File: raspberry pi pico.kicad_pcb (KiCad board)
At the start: 2 copper layers, 51.5 x 20.6 mm, 2 parts, among them J1 USB_OTG, U1 RP2350A

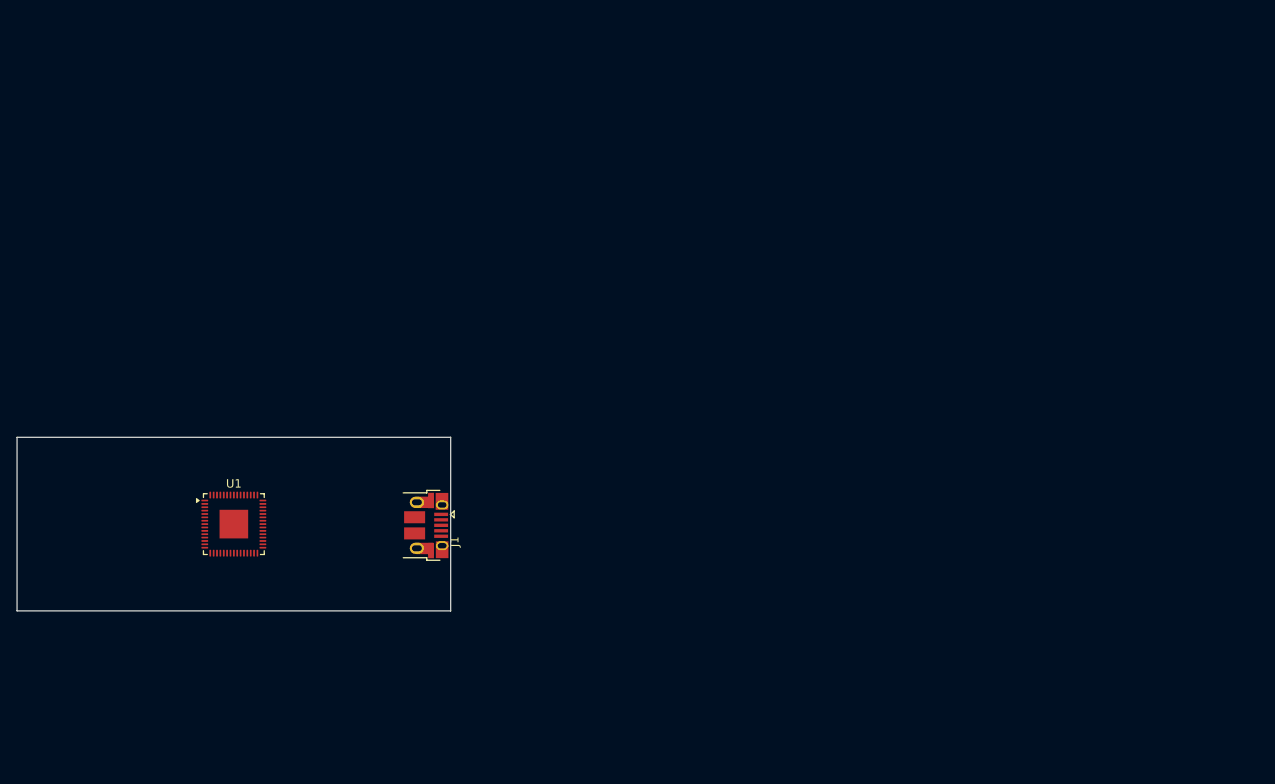
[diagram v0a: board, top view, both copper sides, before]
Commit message: Add files via upload
these files present my progress comparing to the 1st upload
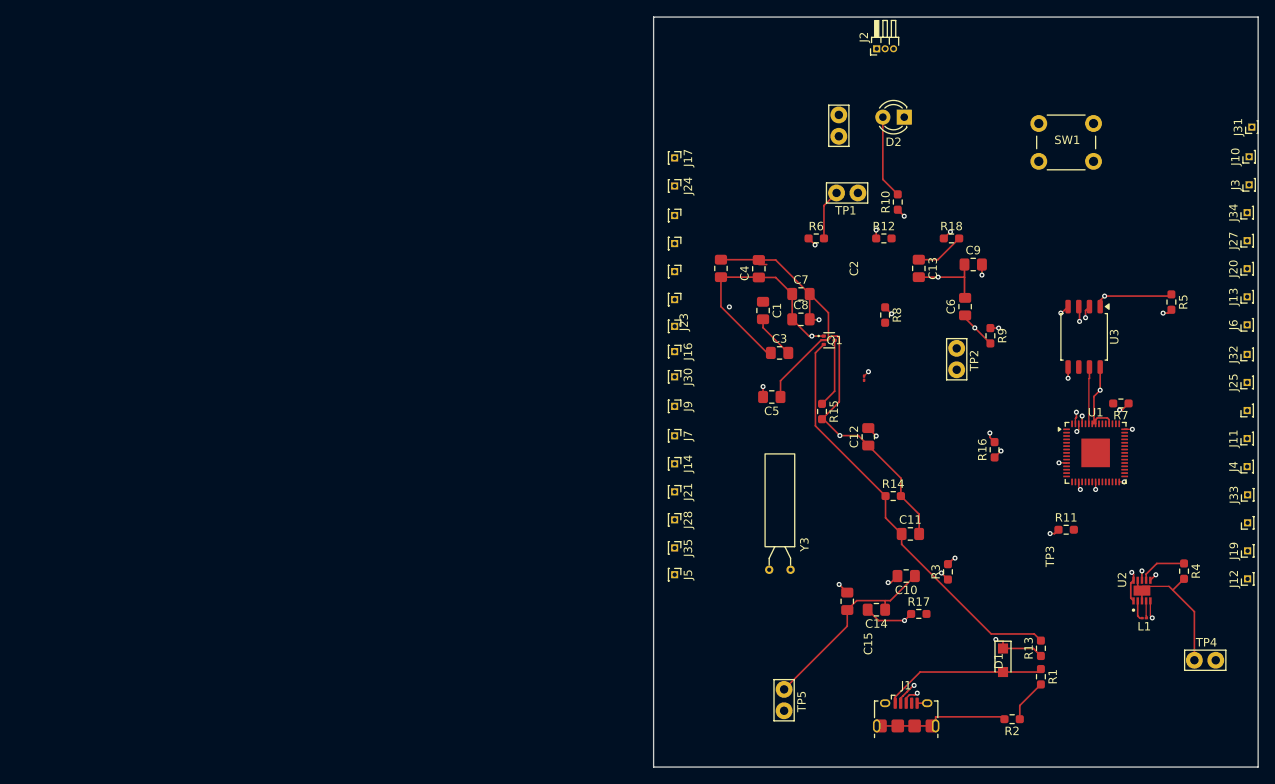
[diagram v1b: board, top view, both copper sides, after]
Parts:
- added C1: 47u, Capacitor_SMD:C_0805_2012Metric_Pad1.18x1.45mm_HandSolder, F.Cu at (213.0, 73.0)
- added C10: 4u7, Capacitor_SMD:C_0805_2012Metric_Pad1.18x1.45mm_HandSolder, F.Cu at (230.0, 104.5)
- added C11: 1n, Capacitor_SMD:C_0805_2012Metric_Pad1.18x1.45mm_HandSolder, F.Cu at (230.5, 99.5)
- added C12: 4u7, Capacitor_SMD:C_0805_2012Metric_Pad1.18x1.45mm_HandSolder, F.Cu at (225.5, 88.0)
- added C13: 4u7, Capacitor_SMD:C_0805_2012Metric_Pad1.18x1.45mm_HandSolder, F.Cu at (231.5, 68.0)
- added C14: 15p, Capacitor_SMD:C_0805_2012Metric_Pad1.18x1.45mm_HandSolder, F.Cu at (226.5, 108.5)
- added C15: 15p, Capacitor_SMD:C_0805_2012Metric_Pad1.18x1.45mm_HandSolder, F.Cu at (223.0, 107.5)
- added C2: C, Capacitor_SMD:C_0805_2012Metric_Pad1.18x1.45mm_HandSolder, F.Cu at (208.0, 68.0)
- added C3: 47uF, Capacitor_SMD:C_0805_2012Metric_Pad1.18x1.45mm_HandSolder, F.Cu at (215.0, 78.0)
- added C4: 100nF, Capacitor_SMD:C_0805_2012Metric_Pad1.18x1.45mm_HandSolder, F.Cu at (212.5, 68.0)
- added C5: 47u, Capacitor_SMD:C_0805_2012Metric_Pad1.18x1.45mm_HandSolder, F.Cu at (214.0, 83.2)
- added C6: 47u, Capacitor_SMD:C_0805_2012Metric_Pad1.18x1.45mm_HandSolder, F.Cu at (237.0, 72.5)
- added C7: 47u, Capacitor_SMD:C_0805_2012Metric_Pad1.18x1.45mm_HandSolder, F.Cu at (217.5, 71.0)
- added C8: 100nF, Capacitor_SMD:C_0805_2012Metric_Pad1.18x1.45mm_HandSolder, F.Cu at (217.5, 74.0)
- added C9: 4u7, Capacitor_SMD:C_0805_2012Metric_Pad1.18x1.45mm_HandSolder, F.Cu at (238.0, 67.5)
- added D1: PMEG6010ELR, Diode_SMD:Nexperia_CFP3_SOD-123W, F.Cu at (241.5, 114.5)
- added D2: LED, LED_THT:LED_D3.0mm, F.Cu at (229.8, 50.0)
- added J10: Conn_01x01_Pin, Connector_PinHeader_1.00mm:PinHeader_1x01_P1.00mm_Vertical, F.Cu at (270.7, 54.7)
- added J11: Conn_01x01_Pin, Connector_PinHeader_1.00mm:PinHeader_1x01_P1.00mm_Vertical, F.Cu at (270.5, 88.2)
- added J12: Conn_01x01_Pin, Connector_PinHeader_1.00mm:PinHeader_1x01_P1.00mm_Vertical, F.Cu at (270.6, 104.8)
- added J13: Conn_01x01_Pin, Connector_PinHeader_1.00mm:PinHeader_1x01_P1.00mm_Vertical, F.Cu at (270.5, 71.3)
- added J14: Conn_01x01_Pin, Connector_PinHeader_1.00mm:PinHeader_1x01_P1.00mm_Vertical, F.Cu at (202.5, 91.2)
- added J15: Conn_01x01_Pin, Connector_PinHeader_1.00mm:PinHeader_1x01_P1.00mm_Vertical, F.Cu at (202.5, 65.0)
- added J16: Conn_01x01_Pin, Connector_PinHeader_1.00mm:PinHeader_1x01_P1.00mm_Vertical, F.Cu at (202.5, 77.8)
- added J17: Conn_01x01_Pin, Connector_PinHeader_1.00mm:PinHeader_1x01_P1.00mm_Vertical, F.Cu at (202.5, 54.8)
- added J18: Conn_01x01_Pin, Connector_PinHeader_1.00mm:PinHeader_1x01_P1.00mm_Vertical, F.Cu at (270.5, 84.8)
- added J19: Conn_01x01_Pin, Connector_PinHeader_1.00mm:PinHeader_1x01_P1.00mm_Vertical, F.Cu at (270.6, 101.5)
- added J2: Conn_01x03_Socket, Connector_PinHeader_1.00mm:PinHeader_1x03_P1.00mm_Horizontal, F.Cu at (226.5, 41.9)
- added J20: Conn_01x01_Pin, Connector_PinHeader_1.00mm:PinHeader_1x01_P1.00mm_Vertical, F.Cu at (270.5, 68.0)
- added J21: Conn_01x01_Pin, Connector_PinHeader_1.00mm:PinHeader_1x01_P1.00mm_Vertical, F.Cu at (202.5, 94.5)
- added J22: Conn_01x01_Pin, Connector_PinHeader_1.00mm:PinHeader_1x01_P1.00mm_Vertical, F.Cu at (202.5, 68.3)
- added J23: Conn_01x01_Pin, Connector_PinHeader_1.00mm:PinHeader_1x01_P1.00mm_Vertical, F.Cu at (202.5, 74.8)
- added J24: Conn_01x01_Pin, Connector_PinHeader_1.00mm:PinHeader_1x01_P1.00mm_Vertical, F.Cu at (202.5, 58.2)
- added J25: Conn_01x01_Pin, Connector_PinHeader_1.00mm:PinHeader_1x01_P1.00mm_Vertical, F.Cu at (270.5, 81.5)
- added J26: Conn_01x01_Pin, Connector_PinHeader_1.00mm:PinHeader_1x01_P1.00mm_Vertical, F.Cu at (270.6, 98.2)
- added J27: Conn_01x01_Pin, Connector_PinHeader_1.00mm:PinHeader_1x01_P1.00mm_Vertical, F.Cu at (270.5, 64.7)
- added J28: Conn_01x01_Pin, Connector_PinHeader_1.00mm:PinHeader_1x01_P1.00mm_Vertical, F.Cu at (202.5, 97.8)
- added J29: Conn_01x01_Pin, Connector_PinHeader_1.00mm:PinHeader_1x01_P1.00mm_Vertical, F.Cu at (202.5, 71.7)
- added J3: Conn_01x01_Pin, Connector_PinHeader_1.00mm:PinHeader_1x01_P1.00mm_Vertical, F.Cu at (270.7, 58.0)
- added J30: Conn_01x01_Pin, Connector_PinHeader_1.00mm:PinHeader_1x01_P1.00mm_Vertical, F.Cu at (202.5, 80.8)
- added J31: Conn_01x01_Pin, Connector_PinHeader_1.00mm:PinHeader_1x01_P1.00mm_Vertical, F.Cu at (271.1, 51.2)
- added J32: Conn_01x01_Pin, Connector_PinHeader_1.00mm:PinHeader_1x01_P1.00mm_Vertical, F.Cu at (270.5, 78.2)
- added J33: Conn_01x01_Pin, Connector_PinHeader_1.00mm:PinHeader_1x01_P1.00mm_Vertical, F.Cu at (270.6, 94.8)
- added J34: Conn_01x01_Pin, Connector_PinHeader_1.00mm:PinHeader_1x01_P1.00mm_Vertical, F.Cu at (270.5, 61.3)
- added J35: Conn_01x01_Pin, Connector_PinHeader_1.00mm:PinHeader_1x01_P1.00mm_Vertical, F.Cu at (202.5, 101.2)
- added J4: Conn_01x01_Pin, Connector_PinHeader_1.00mm:PinHeader_1x01_P1.00mm_Vertical, F.Cu at (270.5, 91.5)
- added J5: Conn_01x01_Pin, Connector_PinHeader_1.00mm:PinHeader_1x01_P1.00mm_Vertical, F.Cu at (202.5, 104.3)
- added J6: Conn_01x01_Pin, Connector_PinHeader_1.00mm:PinHeader_1x01_P1.00mm_Vertical, F.Cu at (270.5, 74.7)
- added J7: Conn_01x01_Pin, Connector_PinHeader_1.00mm:PinHeader_1x01_P1.00mm_Vertical, F.Cu at (202.5, 87.8)
- added J8: Conn_01x01_Pin, Connector_PinHeader_1.00mm:PinHeader_1x01_P1.00mm_Vertical, F.Cu at (202.5, 61.7)
- added J9: Conn_01x01_Pin, Connector_PinHeader_1.00mm:PinHeader_1x01_P1.00mm_Vertical, F.Cu at (202.5, 84.3)
- added L1: L, Inductor_SMD:L_01005_0402Metric, F.Cu at (258.3, 109.5)
- added L2: 3u3, Inductor_SMD:L_01005_0402Metric, F.Cu at (225.0, 81.0)
- added Q1: DMG1012T, Package_TO_SOT_SMD:SOT-523, F.Cu at (220.9, 76.5)
- added R1: 5K, Resistor_SMD:R_0603_1608Metric_Pad0.98x0.95mm_HandSolder, F.Cu at (246.0, 116.5)
- added R10: 470, Resistor_SMD:R_0603_1608Metric_Pad0.98x0.95mm_HandSolder, F.Cu at (229.0, 60.1)
- added R11: 100, Resistor_SMD:R_0603_1608Metric_Pad0.98x0.95mm_HandSolder, F.Cu at (249.0, 99.0)
- added R12: 100, Resistor_SMD:R_0603_1608Metric_Pad0.98x0.95mm_HandSolder, F.Cu at (227.3, 64.4)
- added R13: 100K, Resistor_SMD:R_0603_1608Metric_Pad0.98x0.95mm_HandSolder, F.Cu at (246.0, 113.1)
- added R14: 100K, Resistor_SMD:R_0603_1608Metric_Pad0.98x0.95mm_HandSolder, F.Cu at (228.5, 95.0)
- added R15: 100K, Resistor_SMD:R_0603_1608Metric_Pad0.98x0.95mm_HandSolder, F.Cu at (220.0, 85.0)
- added R16: 200R, Resistor_SMD:R_0603_1608Metric_Pad0.98x0.95mm_HandSolder, F.Cu at (240.5, 89.5)
- added R17: 1K, Resistor_SMD:R_0603_1608Metric_Pad0.98x0.95mm_HandSolder, F.Cu at (231.5, 109.0)
- added R18: 1, Resistor_SMD:R_0603_1608Metric_Pad0.98x0.95mm_HandSolder, F.Cu at (235.4, 64.4)
- added R2: 10K, Resistor_SMD:R_0603_1608Metric_Pad0.98x0.95mm_HandSolder, F.Cu at (242.6, 121.5)
- added R3: 100K, Resistor_SMD:R_0603_1608Metric_Pad0.98x0.95mm_HandSolder, F.Cu at (235.0, 104.0)
- added R4: 100K, Resistor_SMD:R_0603_1608Metric_Pad0.98x0.95mm_HandSolder, F.Cu at (263.0, 103.9)
- added R5: R, Resistor_SMD:R_0603_1608Metric_Pad0.98x0.95mm_HandSolder, F.Cu at (261.5, 72.0)
- added R6: 1K, Resistor_SMD:R_0603_1608Metric_Pad0.98x0.95mm_HandSolder, F.Cu at (219.3, 64.4)
- added R7: 27, Resistor_SMD:R_0603_1608Metric_Pad0.98x0.95mm_HandSolder, F.Cu at (255.5, 84.0)
- added R8: 27, Resistor_SMD:R_0603_1608Metric_Pad0.98x0.95mm_HandSolder, F.Cu at (227.5, 73.5)
- added R9: 100K, Resistor_SMD:R_0603_1608Metric_Pad0.98x0.95mm_HandSolder, F.Cu at (240.0, 76.0)
- added SW1: SW_Push, Button_Switch_THT:SW_PUSH_6mm, F.Cu at (245.8, 50.8)
- added TP1: TestPoint, TestPoint:TestPoint_Bridge_Pitch2.54mm_Drill1.0mm, F.Cu at (221.7, 59.0)
- added TP2: TestPoint, TestPoint:TestPoint_Bridge_Pitch2.54mm_Drill1.0mm, F.Cu at (236.0, 80.0)
- added TP3: TestPoint, TestPoint:TestPoint_Bridge_Pitch2.54mm_Drill1.0mm, F.Cu at (222.0, 52.3)
- added TP4: TestPoint, TestPoint:TestPoint_Bridge_Pitch2.54mm_Drill1.0mm, F.Cu at (266.8, 114.5)
- added TP5: TestPoint, TestPoint:TestPoint_Bridge_Pitch2.54mm_Drill1.0mm, F.Cu at (215.5, 120.5)
- added U2: RT6150B-33GQW, RT6150B-33GQW:SON50P250X250X80-11N, F.Cu at (258.0, 106.2)
- added U3: W25Q32JVSS, Package_SO:SOIC-8_5.3x5.3mm_P1.27mm, F.Cu at (251.1, 76.1)
- added Y3: Crystal, Crystal:Crystal_AT310_D3.0mm_L10.0mm_Horizontal, F.Cu at (216.3, 103.8)
- J1: footprint Connector_USB:USB_Micro-B_Amphenol_10103594-0001LF_Horizontal -> Connector_USB:USB_Micro-B_Amphenol_10118194_Horizontal
- moved U1 102.7 mm to (252.5, 89.9)
- moved J1 61.3 mm to (230.0, 121.0), turned to 0 degrees
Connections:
- J1 pad 1: unconnected-(J1-VBUS-Pad1) -> /VBUS
- J1 pad 2: unconnected-(J1-D--Pad2) -> /D-
- J1 pad 3: unconnected-(J1-D+-Pad3) -> /D+
- J1 pad 5: unconnected-(J1-GND-Pad5) -> GND
- J1 pad SH: unconnected-(J1-Shield-PadSH) -> GND
- U1 pad 1: Net-(U1-IOVDD-Pad1) -> /3V3
- U1 pad 10: unconnected-(U1-GPIO7-Pad10) -> Net-(J11-Pin_1)
- U1 pad 11: Net-(U1-IOVDD-Pad1) -> /3V3
- U1 pad 12: unconnected-(U1-GPIO8-Pad12) -> Net-(J12-Pin_1)
- U1 pad 13: unconnected-(U1-GPIO9-Pad13) -> Net-(J17-Pin_1)
- U1 pad 14: unconnected-(U1-GPIO10-Pad14) -> Net-(J16-Pin_1)
- U1 pad 15: unconnected-(U1-GPIO11-Pad15) -> Net-(J15-Pin_1)
- U1 pad 16: unconnected-(U1-GPIO12-Pad16) -> Net-(J14-Pin_1)
- U1 pad 17: unconnected-(U1-GPIO13-Pad17) -> Net-(J13-Pin_1)
- U1 pad 18: unconnected-(U1-GPIO14-Pad18) -> Net-(J26-Pin_1)
- U1 pad 19: unconnected-(U1-GPIO15-Pad19) -> Net-(J29-Pin_1)
- U1 pad 2: unconnected-(U1-GPIO0-Pad2) -> Net-(J34-Pin_1)
- U1 pad 20: Net-(U1-IOVDD-Pad1) -> /3V3
- U1 pad 21: unconnected-(U1-XIN-Pad21) -> Net-(U1-XIN)
- U1 pad 22: unconnected-(U1-XOUT-Pad22) -> Net-(U1-XOUT)
- U1 pad 23: Net-(U1-DVDD-Pad23) -> /1V1
- U1 pad 24: unconnected-(U1-SWCLK-Pad24) -> /sc
- U1 pad 25: unconnected-(U1-SWDIO-Pad25) -> /sd
- U1 pad 26: unconnected-(U1-RUN-Pad26) -> Net-(J30-Pin_1)
- U1 pad 27: unconnected-(U1-GPIO16-Pad27) -> Net-(J10-Pin_1)
- U1 pad 28: unconnected-(U1-GPIO17-Pad28) -> Net-(J32-Pin_1)
- U1 pad 29: unconnected-(U1-GPIO18-Pad29) -> Net-(J28-Pin_1)
- U1 pad 3: unconnected-(U1-GPIO1-Pad3) -> Net-(J24-Pin_1)
- U1 pad 30: Net-(U1-IOVDD-Pad1) -> /3V3
- U1 pad 31: unconnected-(U1-GPIO19-Pad31) -> Net-(J7-Pin_1)
- U1 pad 32: unconnected-(U1-GPIO20-Pad32) -> Net-(J6-Pin_1)
- U1 pad 33: unconnected-(U1-GPIO21-Pad33) -> Net-(J5-Pin_1)
- U1 pad 34: unconnected-(U1-GPIO22-Pad34) -> Net-(J4-Pin_1)
- U1 pad 35: unconnected-(U1-GPIO23-Pad35) -> GND
- U1 pad 36: unconnected-(U1-GPIO24-Pad36) -> Net-(J18-Pin_1)
- U1 pad 37: unconnected-(U1-GPIO25-Pad37) -> Net-(J31-Pin_1)
- U1 pad 38: Net-(U1-IOVDD-Pad1) -> /3V3
- U1 pad 39: Net-(U1-DVDD-Pad23) -> /1V1
- U1 pad 4: unconnected-(U1-GPIO2-Pad4) -> Net-(J25-Pin_1)
- U1 pad 40: unconnected-(U1-GPIO26/ADC0-Pad40) -> Net-(J22-Pin_1)
- U1 pad 41: unconnected-(U1-GPIO27/ADC1-Pad41) -> Net-(J21-Pin_1)
- U1 pad 42: unconnected-(U1-GPIO28/ADC2-Pad42) -> Net-(J20-Pin_1)
- U1 pad 43: unconnected-(U1-GPIO29/ADC3-Pad43) -> Net-(J19-Pin_1)
- U1 pad 44: unconnected-(U1-ADC_AVDD-Pad44) -> Net-(U1-ADC_AVDD)
- U1 pad 45: Net-(U1-IOVDD-Pad1) -> /3V3
- U1 pad 46: unconnected-(U1-VREG_AVDD-Pad46) -> Net-(U1-VREG_AVDD)
- U1 pad 47: unconnected-(U1-VREG_PGND-Pad47) -> GND
- U1 pad 48: unconnected-(U1-VREG_LX-Pad48) -> Net-(U1-VREG_LX)
- U1 pad 49: unconnected-(U1-VREG_VIN-Pad49) -> /3V3
- U1 pad 5: unconnected-(U1-GPIO3-Pad5) -> Net-(J33-Pin_1)
- U1 pad 50: unconnected-(U1-VREG_FB-Pad50) -> /1V1
- U1 pad 51: unconnected-(U1-USB_DM-Pad51) -> Net-(U1-USB_DM)
- U1 pad 52: unconnected-(U1-USB_DP-Pad52) -> Net-(U1-USB_DP)
- U1 pad 53: unconnected-(U1-USB_OTP_VDD-Pad53) -> /3V3
- U1 pad 54: unconnected-(U1-QSPI_IOVDD-Pad54) -> /3V3
- U1 pad 55: unconnected-(U1-QSPI_SD3-Pad55) -> Net-(U1-QSPI_SD3)
- U1 pad 56: unconnected-(U1-QSPI_SCLK-Pad56) -> Net-(U1-QSPI_SCLK)
- U1 pad 57: unconnected-(U1-QSPI_SD0-Pad57) -> Net-(U1-QSPI_SD0)
- U1 pad 58: unconnected-(U1-QSPI_SD2-Pad58) -> Net-(U1-QSPI_SD2)
- U1 pad 59: unconnected-(U1-QSPI_SD1-Pad59) -> Net-(U1-QSPI_SD1)
- U1 pad 6: Net-(U1-DVDD-Pad23) -> /1V1
- U1 pad 60: unconnected-(U1-~{QSPI_SS}-Pad60) -> Net-(U1-~{QSPI_SS})
- U1 pad 61: unconnected-(U1-GND-Pad61) -> GND
- U1 pad 7: unconnected-(U1-GPIO4-Pad7) -> Net-(J27-Pin_1)
- U1 pad 8: unconnected-(U1-GPIO5-Pad8) -> Net-(J9-Pin_1)
- U1 pad 9: unconnected-(U1-GPIO6-Pad9) -> Net-(J35-Pin_1)
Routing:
- net GND: track 0.00 -> 337.0 mm, vias 0 -> 4
- net /3V3: track 0.00 -> 172.8 mm, vias 0 -> 10
- net Net-(U1-VREG_AVDD): track 0.00 -> 122.1 mm, vias 0 -> 2
- net Net-(D1-K): track 0.00 -> 102.8 mm, vias 0 -> 5
- net Net-(J17-Pin_1): track 0.00 -> 92.6 mm
- net Net-(J2-Pin_3): track 0.00 -> 66.5 mm, vias 0 -> 1
- net /1V1: track 0.00 -> 64.0 mm, vias 0 -> 4
- net Net-(Q1-S): track 0.00 -> 49.7 mm
- net /D-: track 0.00 -> 49.1 mm, vias 0 -> 2
- net /D+: track 0.00 -> 47.5 mm, vias 0 -> 2
- net Net-(U1-~{QSPI_SS}): track 0.00 -> 47.5 mm, vias 0 -> 2
- net Net-(J31-Pin_1): track 0.00 -> 46.8 mm, vias 0 -> 1
- net Net-(R6-Pad2): track 0.00 -> 40.0 mm
- net Net-(J25-Pin_1): track 0.00 -> 33.3 mm
- net /ADC_VREF: track 0.00 -> 28.3 mm, vias 0 -> 2
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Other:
- board size 51.5 x 20.6 mm -> 71.8 x 89.1 mm
- copper layers 2 -> 4
